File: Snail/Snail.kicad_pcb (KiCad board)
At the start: 2 copper layers, 88 parts, among them J1 Arduino Nano SuperMini, Q1 MMBT3904, SW0 SW_Push, SW1 SW_Push, SW2 SW_Push, SW3 SW_Push

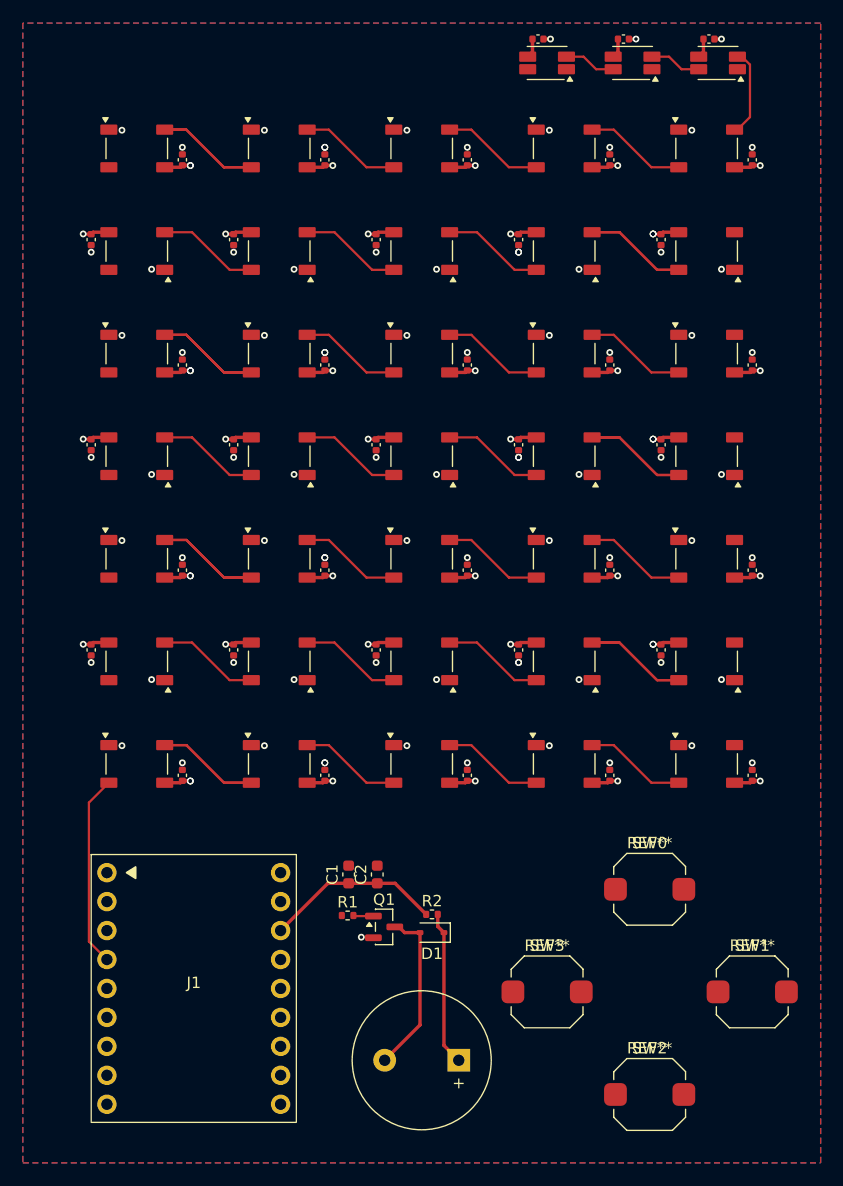
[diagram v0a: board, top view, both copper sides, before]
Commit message: Finish layout & routing
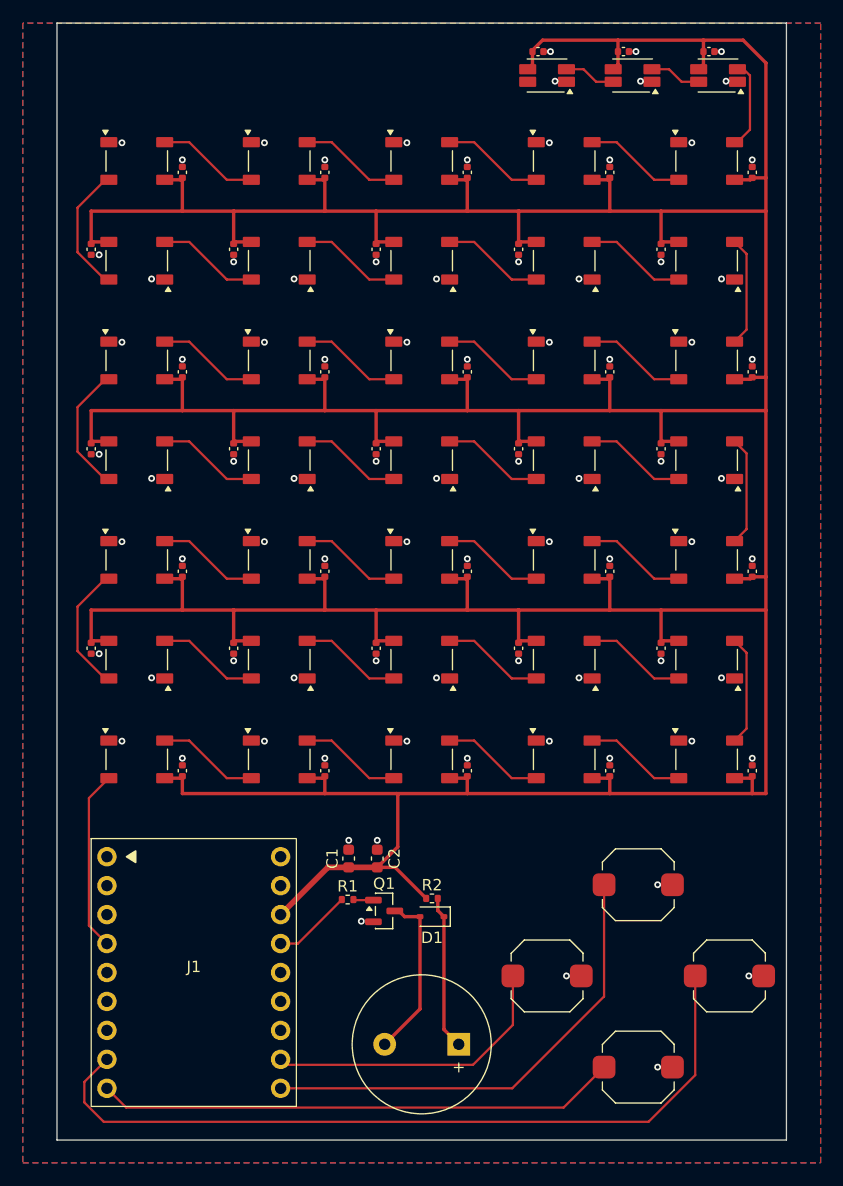
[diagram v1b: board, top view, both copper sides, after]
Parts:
- moved SW2 2.60 mm to (114.0, 126.6)
- moved SW1 2.44 mm to (122.0, 118.6)
- moved BZ1 1.40 mm to (98.2, 124.6)
- moved C1 1.40 mm to (88.6, 108.3)
- moved C2 1.40 mm to (91.1, 108.3)
- moved J1 1.40 mm to (75.0, 118.3)
- moved R2 1.40 mm to (95.9, 111.8)
- moved SW3 1.40 mm to (106.0, 118.6)
- moved D1 1.40 mm to (95.9, 113.4)
- moved Q1 1.40 mm to (91.7, 112.9)
- moved R1 1.40 mm to (88.5, 111.9)
- moved C130 1.10 mm to (74.0, 48.1)
- moved C131 1.10 mm to (86.5, 48.1)
- moved C132 1.10 mm to (99.0, 48.1)
- moved C133 1.10 mm to (111.5, 48.1)
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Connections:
- J1 pad 10: unconnected-(J1-Pin_10-Pad10) -> /KEY_0
- J1 pad 11: unconnected-(J1-Pin_11-Pad11) -> /KEY_3
- J1 pad 12: /KEY_0 -> unconnected-(J1-Pin_12-Pad12)
- J1 pad 13: /KEY_1 -> unconnected-(J1-Pin_13-Pad13)
- J1 pad 14: /KEY_2 -> unconnected-(J1-Pin_14-Pad14)
- J1 pad 15: /KEY_3 -> /BUZZER
- J1 pad 6: /BUZZER -> unconnected-(J1-Pin_6-Pad6)
- J1 pad 8: unconnected-(J1-Pin_8-Pad8) -> /KEY_1
- J1 pad 9: unconnected-(J1-Pin_9-Pad9) -> /KEY_2
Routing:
- net +5V: track 102.3 -> 490.7 mm, vias 42 -> 0
- net /KEY_1: track 0.00 -> 69.3 mm
- net /KEY_2: track 0.00 -> 45.8 mm
- net /KEY_0: track 0.00 -> 41.5 mm
- net /KEY_3: track 0.00 -> 26.3 mm
- net Net-(D129-DOUT): track 0.00 -> 11.4 mm
- net Net-(D119-DOUT): track 0.00 -> 11.4 mm
- net Net-(D109-DOUT): track 0.00 -> 11.4 mm
- net Net-(D114-DOUT): track 0.00 -> 9.62 mm
- net Net-(D104-DOUT): track 0.00 -> 9.62 mm
- net Net-(D124-DOUT): track 0.00 -> 9.62 mm
- net Net-(D115-DOUT): track 17.9 -> 8.97 mm
- net Net-(D110-DOUT): track 17.9 -> 8.97 mm
- net Net-(D105-DOUT): track 17.9 -> 8.97 mm
- net Net-(D100-DOUT): track 17.9 -> 8.97 mm
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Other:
- board outline added: 64 x 98 mm
